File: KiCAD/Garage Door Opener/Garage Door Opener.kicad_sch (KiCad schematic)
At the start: 8 parts, among them J1 Screw_Terminal_01x03, J3 Conn_01x02_Pin, K1 JQC-3FF-S-Z, Q1 S8550, SW1 SW_Push_Dual, U1 ESP32-S3-DevKitC

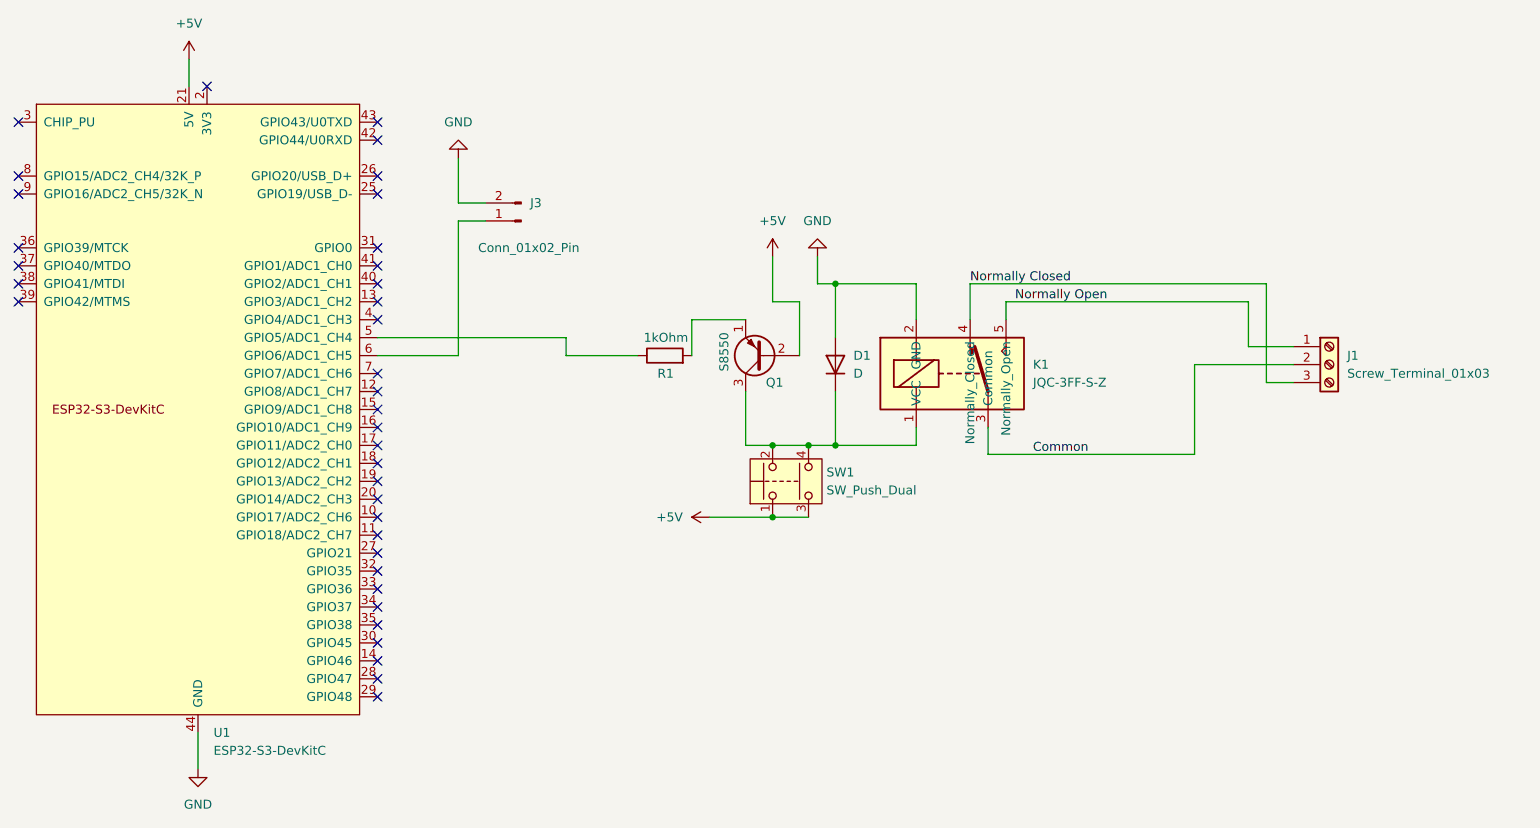
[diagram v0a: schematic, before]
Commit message: Updated board design
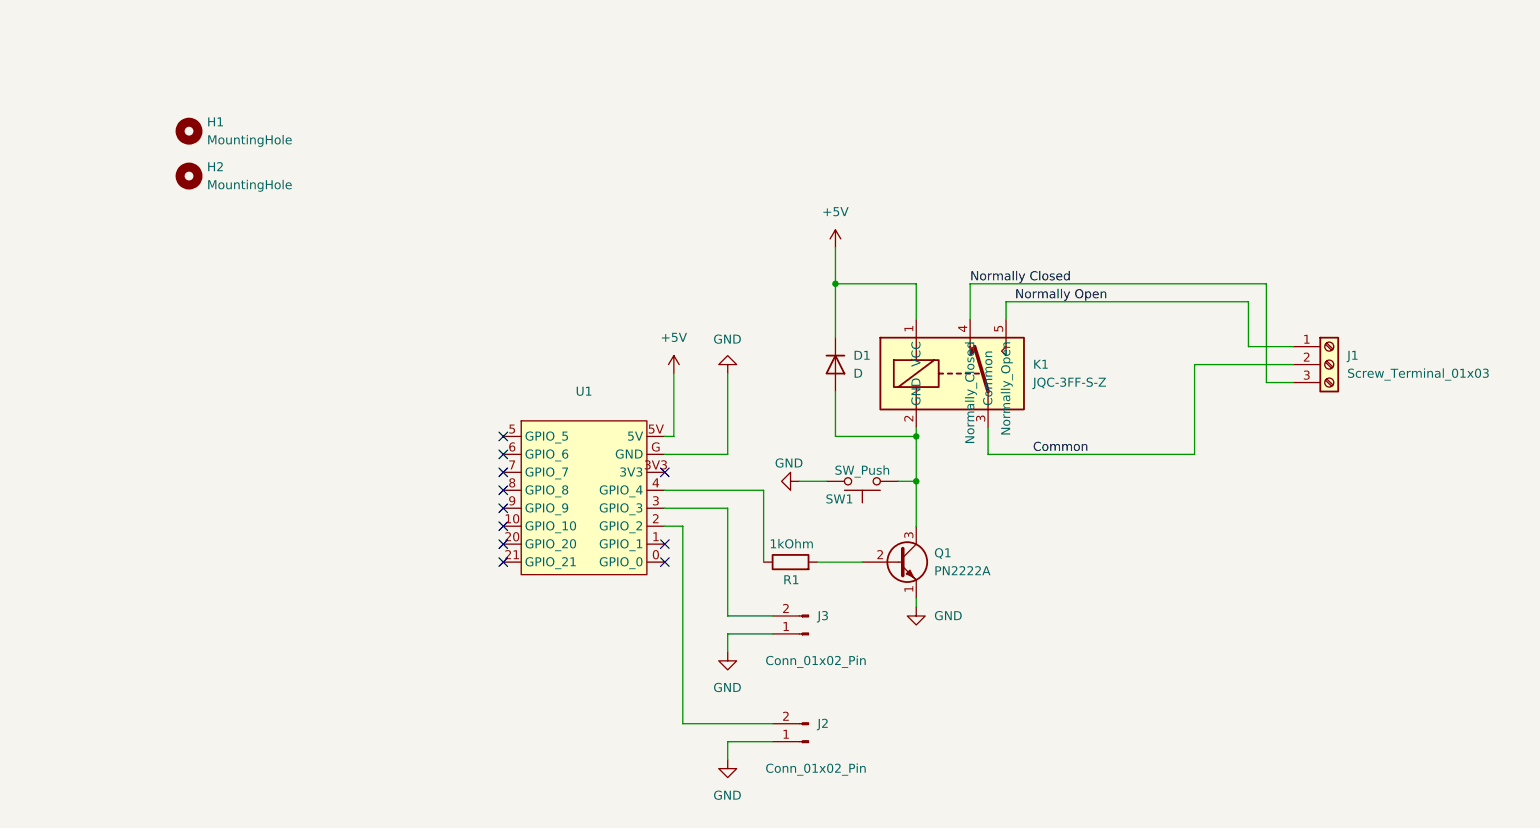
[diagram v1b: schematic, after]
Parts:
- removed Q1: S8550, Package_TO_SOT_SMD:SOT-23, symbol Transistor_BJT:S8550
- removed U1: ESP32-S3-DevKitC, Custom Footprints:YD-ESP32-S3, symbol PCM_Espressif:ESP32-S3-DevKitC
- added H1, H2: MountingHole, MountingHole:MountingHole_3.5mm, symbol Mechanical:MountingHole
- added J2: Conn_01x02_Pin, Connector_PinHeader_2.54mm:PinHeader_1x02_P2.54mm_Vertical, symbol Connector:Conn_01x02_Pin
- added Q1: PN2222A, Package_TO_SOT_THT:TO-92_Inline, symbol Transistor_BJT:PN2222A
- added U1: ~, esp32-homespan-garagedoor-opener:ESP32-C3 Super Micro, symbol esp32-homespan-garagedoor-opener:ESP32-C3_Super_Mini
- D1: footprint Diode_SMD:D_MiniMELF -> Diode_THT:D_DO-35_SOD27_P7.62mm_Horizontal
- R1: footprint Resistor_SMD:R_0805_2012Metric -> Resistor_THT:R_Axial_DIN0207_L6.3mm_D2.5mm_P7.62mm_Horizontal
- SW1: value SW_Push_Dual -> SW_Push; symbol Switch:SW_Push_Dual -> Switch:SW_Push
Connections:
- net +5V: now also D1.1 (K), K1.1 (VCC), U1.5V; no longer SW1.1, SW1.3
- net GND: now also J3.1 (Pin_1), SW1.2, J2.1 (Pin_1), Q1.1 (E), U1.G (GND); no longer D1.2 (A), J3.2 (Pin_2), K1.2 (GND)
- net at R1.1: now also U1.4 (GPIO_4)
- net at R1.2: now also Q1.2 (B)
- new net: D1.2 (A), K1.2 (GND), Q1.3 (C), SW1.1
- new net: J2.2 (Pin_2), U1.2 (GPIO_2)
- new net: J3.2 (Pin_2), U1.3 (GPIO_3)
- no-connect marks 36 -> 11
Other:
- moved on the sheet: D1, J3, R1
